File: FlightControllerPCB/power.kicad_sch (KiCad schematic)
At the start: 12 parts, among them J4 USB_C_Receptacle_USB2.0_16P, U13 D3V3XA4B10LP, U16 AMS1117-3.3, U2 AP2112K-1.8

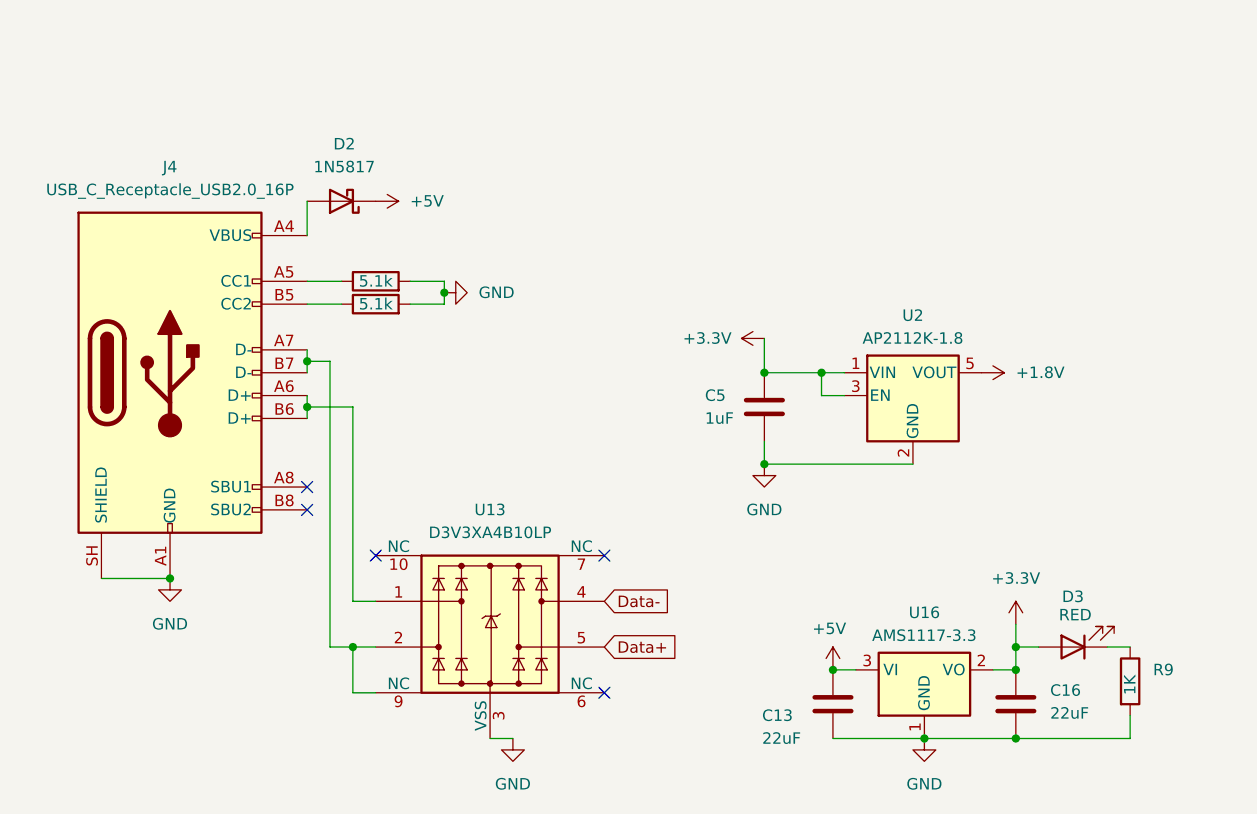
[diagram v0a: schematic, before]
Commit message: Power circuit
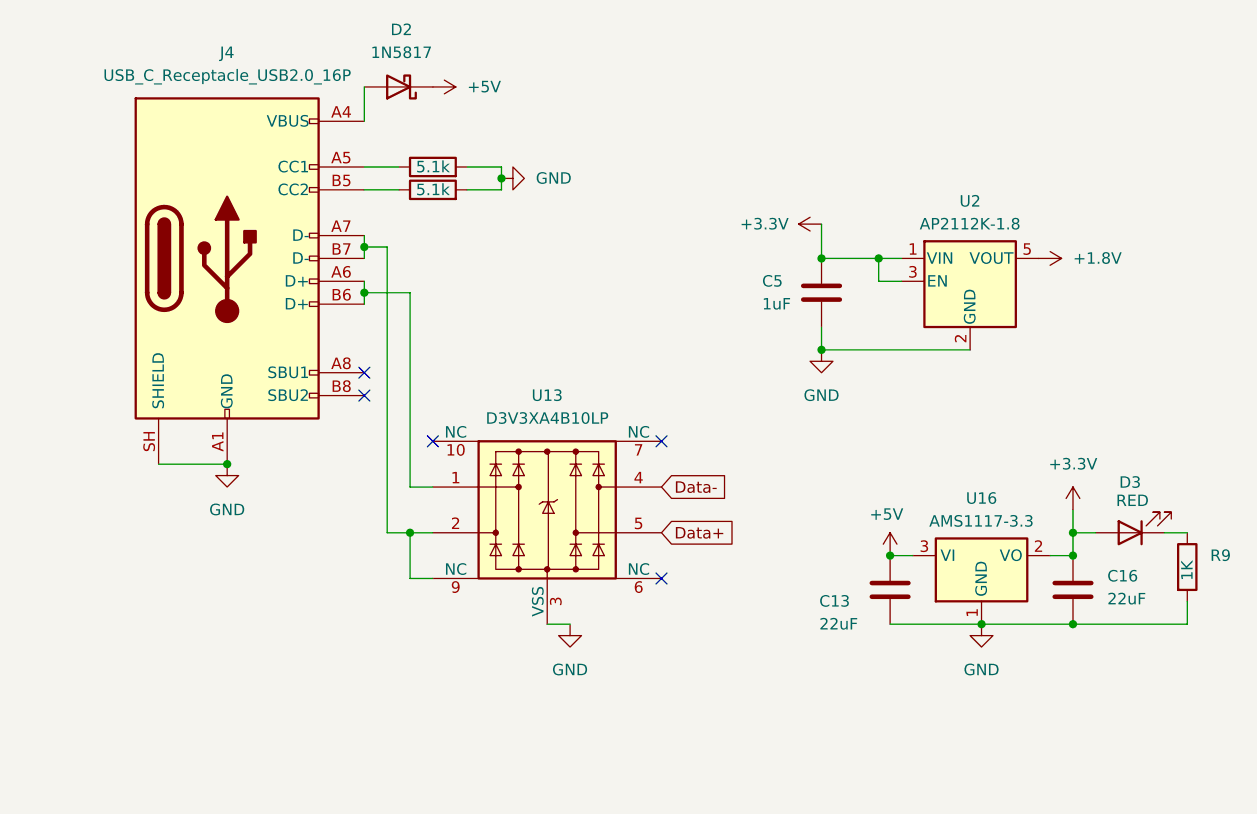
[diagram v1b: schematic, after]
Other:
- moved on the sheet: C13, C16, C5, D2, D3, J4, R9, U13, U16, U2
